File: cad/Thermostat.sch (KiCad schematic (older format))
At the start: 14 parts, among them J1 Screw_Terminal_01x03, J2 Screw_Terminal_01x03, J3 Screw_Terminal_01x02, K1 RSM822, SW1 Rotary_Encoder_Switch, U1 WeMos_mini, U2 ILI9341_LCD_Breakout

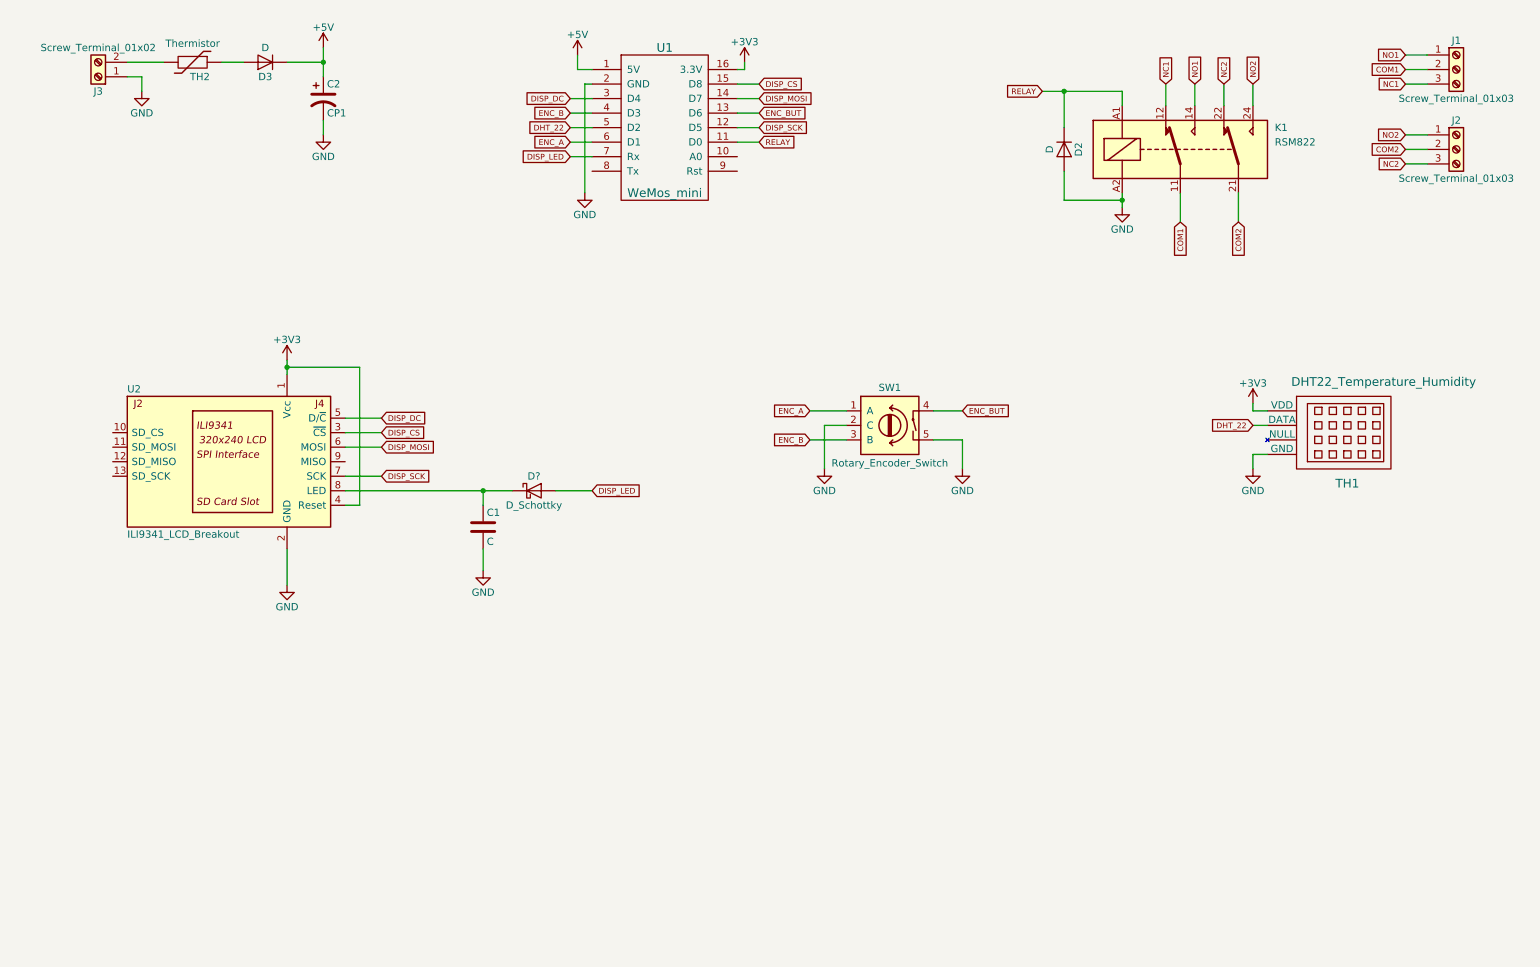
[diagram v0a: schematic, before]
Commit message: PCB
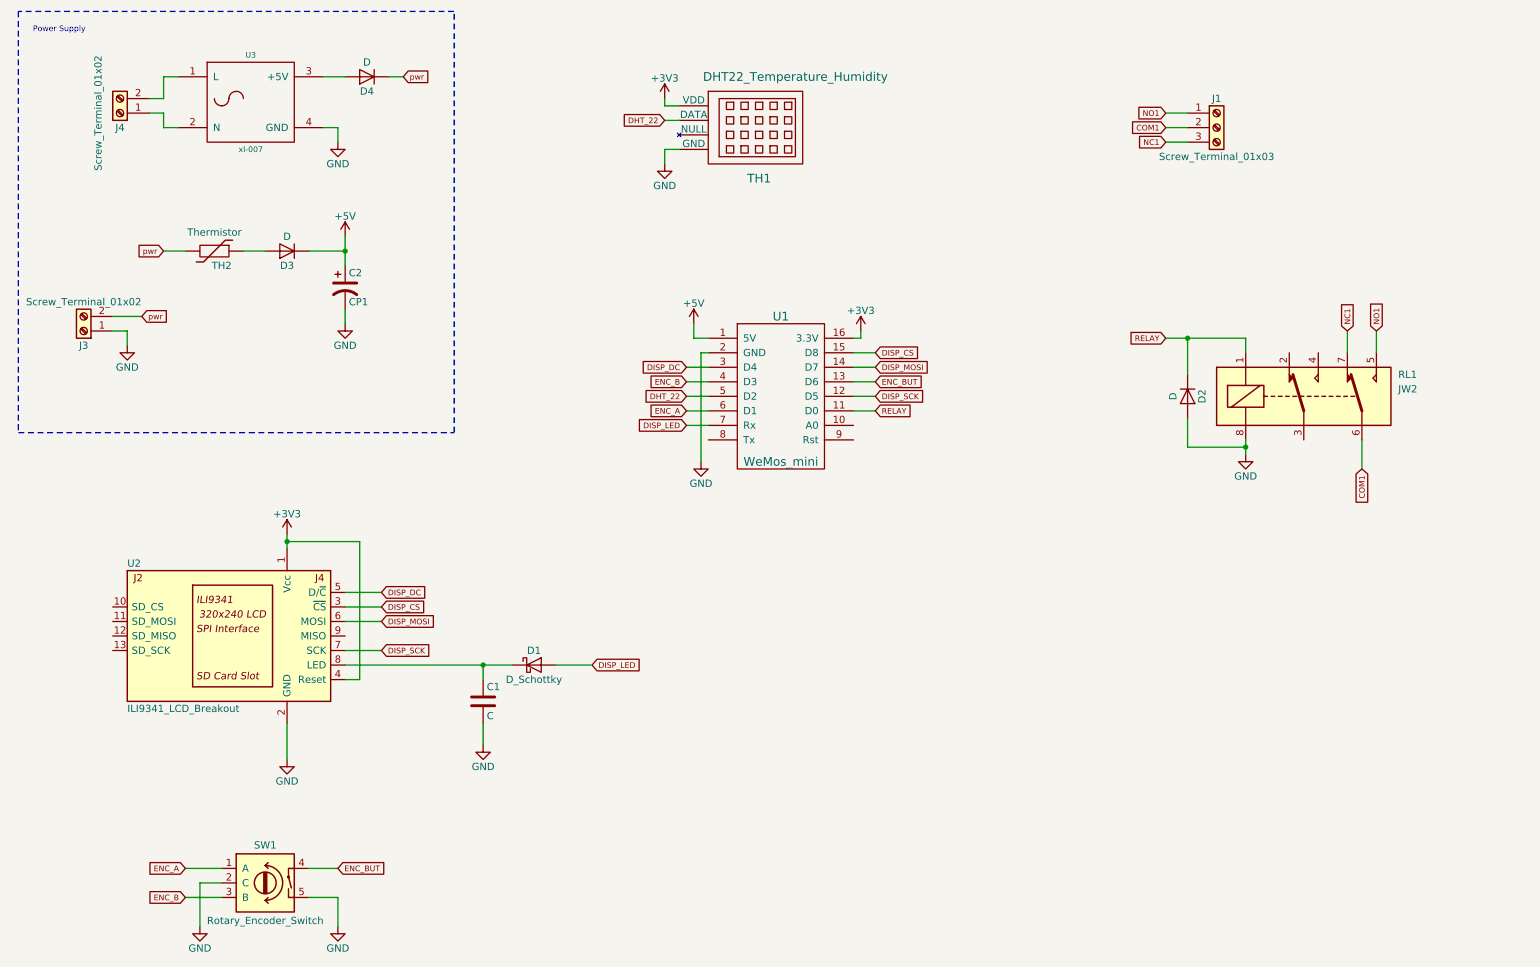
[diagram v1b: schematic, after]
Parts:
- removed J2: Screw_Terminal_01x03, symbol Screw_Terminal_01x03
- removed K1: RSM822, Relays_THT:Relay_DPDT_Finder_40.52, symbol RSM822
- added D4: D, Resistors_Universal:Resistor_SMD+THTuniversal_0805to2512_HandSoldering, symbol D
- added J4: Screw_Terminal_01x02, Connectors_Phoenix:PhoenixContact_MC-GF_02x5.08mm_Angled_ThreadedFlange, symbol Screw_Terminal_01x02
- added RL1: JW2, Relays_THT:Relay_DPDT_Omron_G5V-2, symbol JW2
- added U3: xl-007, xl007:xl007, symbol xl-007
- C1, C2, D2, D3, TH2: footprint (none) -> Resistors_Universal:Resistor_SMD+THTuniversal_0805to2512_HandSoldering
- D1: renamed from D?; footprint (none) -> Resistors_Universal:Resistor_SMD+THTuniversal_0805to2512_HandSoldering
- J1: footprint (none) -> Connectors_Phoenix:PhoenixContact_MC-GF_03x5.08mm_Angled_ThreadedFlange
- J3: footprint (none) -> Connectors_Phoenix:PhoenixContact_MC-GF_02x5.08mm_Angled_ThreadedFlange
- SW1: footprint (none) -> sparkfun:SF-ROTARY-ENCODER
- TH1: footprint (none) -> Sensors:DHT22_Temperature_Humidity
- U1: footprint (none) -> wemos_d1_mini:D1_mini_board
- U2: footprint (none) -> ILI9431:ILI9431 2,8 TFT
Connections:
- net COM1: now also RL1.6
- net GND: now also RL1.8, U3.4 (GND)
- net NC1: now also RL1.7
- net NO1: now also RL1.5
- net RELAY: now also RL1.1
- net pwr: now reaches J3.2 (Pin_2), TH2.2
- net pwr: now also D4.1 (K)
- new net: J4.2 (Pin_2), U3.1 (L)
- new net: J4.1 (Pin_1), U3.2 (N)
- new net: D4.2 (A), U3.3 (+5V)
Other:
- note added: "Power Supply"
- moved on the sheet: C1, C2, D1, D2, D3, J1, J3, SW1, TH1, TH2, U1, U2
